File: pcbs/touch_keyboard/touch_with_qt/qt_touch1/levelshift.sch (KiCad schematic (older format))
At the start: 6 parts, among them U2 cd40109, U3 cd40109

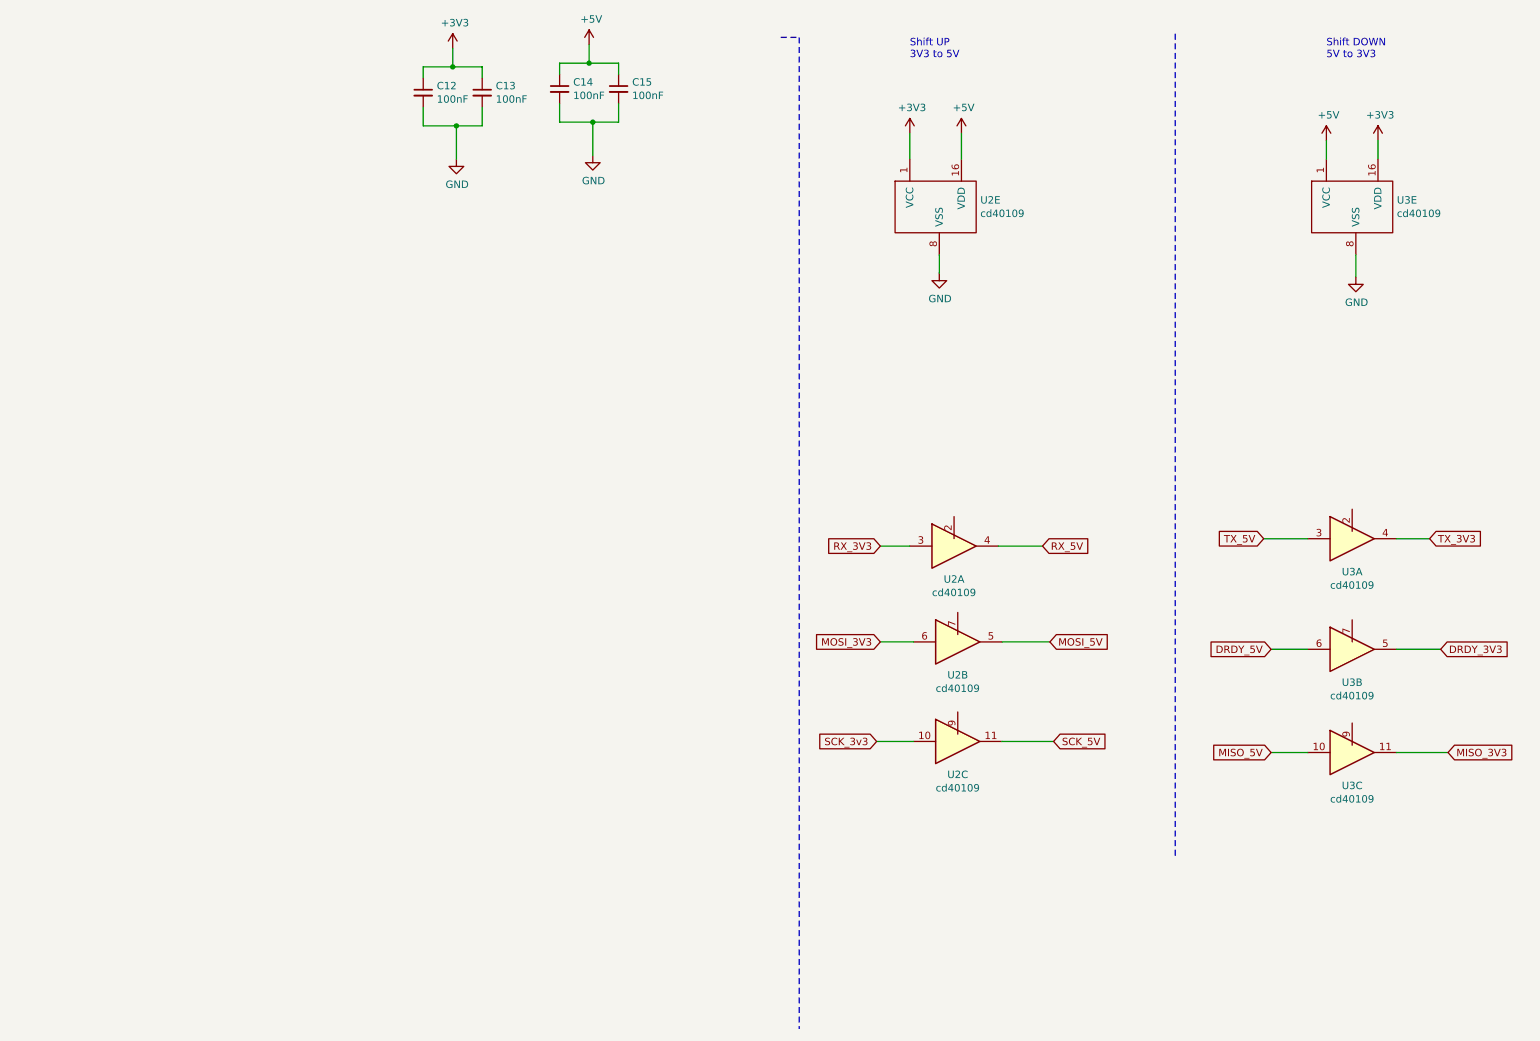
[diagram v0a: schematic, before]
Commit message: Updates
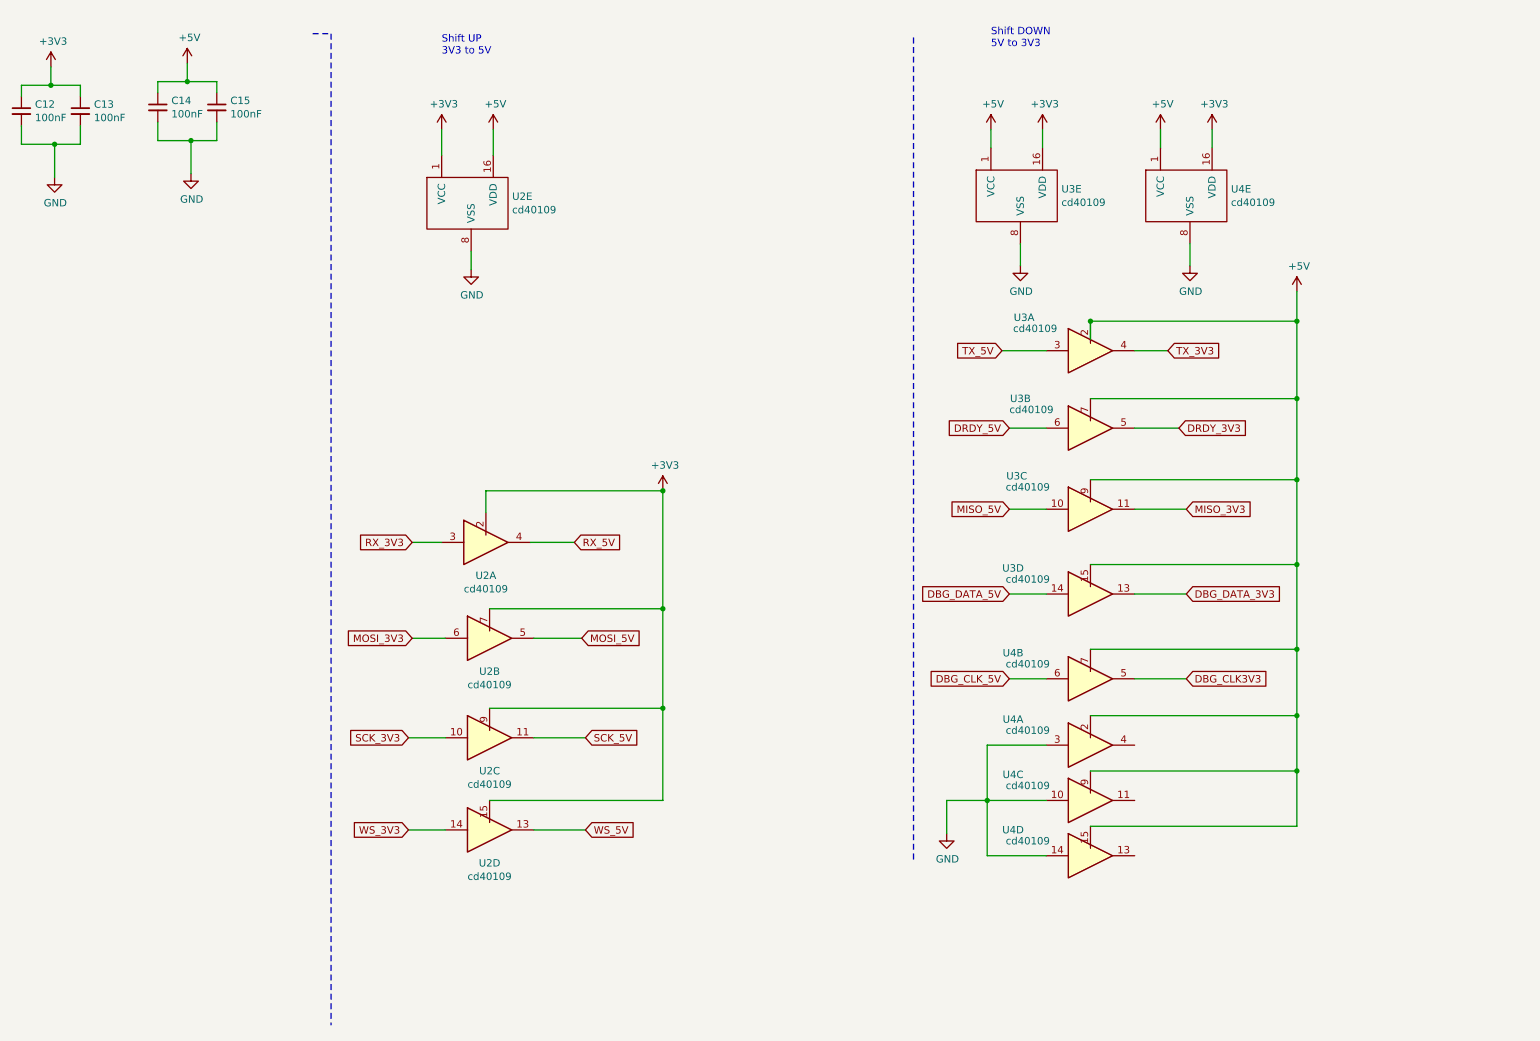
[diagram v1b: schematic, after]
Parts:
- added unit 4 of U2
- added unit 4 of U3
- added U4: cd40109, Package_SO:SOP-24_7.5x15.4mm_P1.27mm, symbol ajm:cd40109
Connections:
- net +3V3: now also U2.2, U2.7, U2.9, U2.15, U4.16 (VDD)
- net +5V: now also U3.2, U3.7, U3.9, U3.15, U4.1 (VCC), U4.15, U4.2, U4.7, U4.9
- net GND: now also U4.10, U4.14, U4.3, U4.8 (VSS)
- net SCK_3v3 renamed SCK_3V3
- new net DBG_CLK3V3: U4.5
- new net DBG_CLK_5V: U4.6
- new net DBG_DATA_3V3: U3.13
- new net DBG_DATA_5V: U3.14
- new net WS_3V3: U2.14
- new net WS_5V: U2.13
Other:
- moved on the sheet: C12, C13, C14, C15, U2A, U2B, U2C, U2E, U3A, U3B, U3C, U3E

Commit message: Updates
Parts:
- U2, U3, U4: footprint Package_SO:SOP-24_7.5x15.4mm_P1.27mm -> Package_SO:SOIC-16W_7.5x10.3mm_P1.27mm
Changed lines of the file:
@@
 F 0 "U2" H 3925 3925 50  0000 C CNN
 F 1 "cd40109" H 3925 3834 50  0000 C CNN
-F 2 "Package_SO:SOP-24_7.5x15.4mm_P1.27mm" H 3725 4450 50  0001 C CNN
+F 2 "Package_SO:SOIC-16W_7.5x10.3mm_P1.27mm" H 3725 4450 50  0001 C CNN
 F 3 "" H 3725 4450 50  0001 C CNN
 	1    3925 4150
@@
 F 0 "U2" H 4103 1846 50  0000 L CNN
 F 1 "cd40109" H 4103 1755 50  0000 L CNN
-F 2 "Package_SO:SOP-24_7.5x15.4mm_P1.27mm" H 3525 2125 50  0001 C CNN
+F 2 "Package_SO:SOIC-16W_7.5x10.3mm_P1.27mm" H 3525 2125 50  0001 C CNN
 F 3 "" H 3525 2125 50  0001 C CNN
 	5    3725 1825
@@
 F 0 "U3" H 7575 3075 50  0000 C CNN
 F 1 "cd40109" H 7650 3000 50  0000 C CNN
-F 2 "Package_SO:SOP-24_7.5x15.4mm_P1.27mm" H 7825 3150 50  0001 C CNN
+F 2 "Package_SO:SOIC-16W_7.5x10.3mm_P1.27mm" H 7825 3150 50  0001 C CNN
 F 3 "" H 7825 3150 50  0001 C CNN
 	1    8025 2850
@@
 F 0 "U3" H 7828 1796 50  0000 L CNN
 F 1 "cd40109" H 7828 1705 50  0000 L CNN
-F 2 "Package_SO:SOP-24_7.5x15.4mm_P1.27mm" H 7250 2075 50  0001 C CNN
+F 2 "Package_SO:SOIC-16W_7.5x10.3mm_P1.27mm" H 7250 2075 50  0001 C CNN
 F 3 "" H 7250 2075 50  0001 C CNN
 	5    7450 1775
@@
 F 0 "U3" H 7550 3575 50  0000 C CNN
 F 1 "cd40109" H 7625 3500 50  0000 C CNN
-F 2 "Package_SO:SOP-24_7.5x15.4mm_P1.27mm" H 7825 3675 50  0001 C CNN
+F 2 "Package_SO:SOIC-16W_7.5x10.3mm_P1.27mm" H 7825 3675 50  0001 C CNN
 F 3 "" H 7825 3675 50  0001 C CNN
 	2    8025 3375
@@
 F 0 "U3" H 7525 4150 50  0000 C CNN
 F 1 "cd40109" H 7600 4075 50  0000 C CNN
-F 2 "Package_SO:SOP-24_7.5x15.4mm_P1.27mm" H 7825 4225 50  0001 C CNN
+F 2 "Package_SO:SOIC-16W_7.5x10.3mm_P1.27mm" H 7825 4225 50  0001 C CNN
 F 3 "" H 7825 4225 50  0001 C CNN
 	3    8025 3925
@@
 F 0 "U2" H 3950 5250 50  0000 C CNN
 F 1 "cd40109" H 3950 5159 50  0000 C CNN
-F 2 "Package_SO:SOP-24_7.5x15.4mm_P1.27mm" H 3750 5775 50  0001 C CNN
+F 2 "Package_SO:SOIC-16W_7.5x10.3mm_P1.27mm" H 3750 5775 50  0001 C CNN
 F 3 "" H 3750 5775 50  0001 C CNN
 	3    3950 5475
@@
 F 0 "U2" H 3950 4575 50  0000 C CNN
 F 1 "cd40109" H 3950 4484 50  0000 C CNN
-F 2 "Package_SO:SOP-24_7.5x15.4mm_P1.27mm" H 3750 5100 50  0001 C CNN
+F 2 "Package_SO:SOIC-16W_7.5x10.3mm_P1.27mm" H 3750 5100 50  0001 C CNN
 F 3 "" H 3750 5100 50  0001 C CNN
 	2    3950 4800
@@
 F 0 "U3" H 7500 4675 50  0000 C CNN
 F 1 "cd40109" H 7600 4600 50  0000 C CNN
-F 2 "Package_SO:SOP-24_7.5x15.4mm_P1.27mm" H 7825 4800 50  0001 C CNN
+F 2 "Package_SO:SOIC-16W_7.5x10.3mm_P1.27mm" H 7825 4800 50  0001 C CNN
 F 3 "" H 7825 4800 50  0001 C CNN
 	4    8025 4500
@@
 F 0 "U4" H 8978 1796 50  0000 L CNN
 F 1 "cd40109" H 8978 1705 50  0000 L CNN
-F 2 "Package_SO:SOP-24_7.5x15.4mm_P1.27mm" H 8400 2075 50  0001 C CNN
+F 2 "Package_SO:SOIC-16W_7.5x10.3mm_P1.27mm" H 8400 2075 50  0001 C CNN
 F 3 "" H 8400 2075 50  0001 C CNN
 	5    8600 1775
@@
 F 0 "U4" H 7500 5250 50  0000 C CNN
 F 1 "cd40109" H 7600 5175 50  0000 C CNN
-F 2 "Package_SO:SOP-24_7.5x15.4mm_P1.27mm" H 7825 5375 50  0001 C CNN
+F 2 "Package_SO:SOIC-16W_7.5x10.3mm_P1.27mm" H 7825 5375 50  0001 C CNN
 F 3 "" H 7825 5375 50  0001 C CNN
 	2    8025 5075
@@
 F 0 "U2" H 3950 5875 50  0000 C CNN
 F 1 "cd40109" H 3950 5784 50  0000 C CNN
-F 2 "Package_SO:SOP-24_7.5x15.4mm_P1.27mm" H 3750 6400 50  0001 C CNN
+F 2 "Package_SO:SOIC-16W_7.5x10.3mm_P1.27mm" H 3750 6400 50  0001 C CNN
 F 3 "" H 3750 6400 50  0001 C CNN
 	4    3950 6100
@@
 F 0 "U4" H 7500 5700 50  0000 C CNN
 F 1 "cd40109" H 7600 5625 50  0000 C CNN
-F 2 "Package_SO:SOP-24_7.5x15.4mm_P1.27mm" H 7825 5825 50  0001 C CNN
+F 2 "Package_SO:SOIC-16W_7.5x10.3mm_P1.27mm" H 7825 5825 50  0001 C CNN
 F 3 "" H 7825 5825 50  0001 C CNN
 	1    8025 5525
@@
 F 0 "U4" H 7500 6075 50  0000 C CNN
 F 1 "cd40109" H 7600 6000 50  0000 C CNN
-F 2 "Package_SO:SOP-24_7.5x15.4mm_P1.27mm" H 7825 6200 50  0001 C CNN
+F 2 "Package_SO:SOIC-16W_7.5x10.3mm_P1.27mm" H 7825 6200 50  0001 C CNN
 F 3 "" H 7825 6200 50  0001 C CNN
 	3    8025 5900
@@
 F 0 "U4" H 7500 6450 50  0000 C CNN
 F 1 "cd40109" H 7600 6375 50  0000 C CNN
-F 2 "Package_SO:SOP-24_7.5x15.4mm_P1.27mm" H 7825 6575 50  0001 C CNN
+F 2 "Package_SO:SOIC-16W_7.5x10.3mm_P1.27mm" H 7825 6575 50  0001 C CNN
 F 3 "" H 7825 6575 50  0001 C CNN
 	4    8025 6275
